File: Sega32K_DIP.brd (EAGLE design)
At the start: 65.7 x 37.9 mm, 4 parts

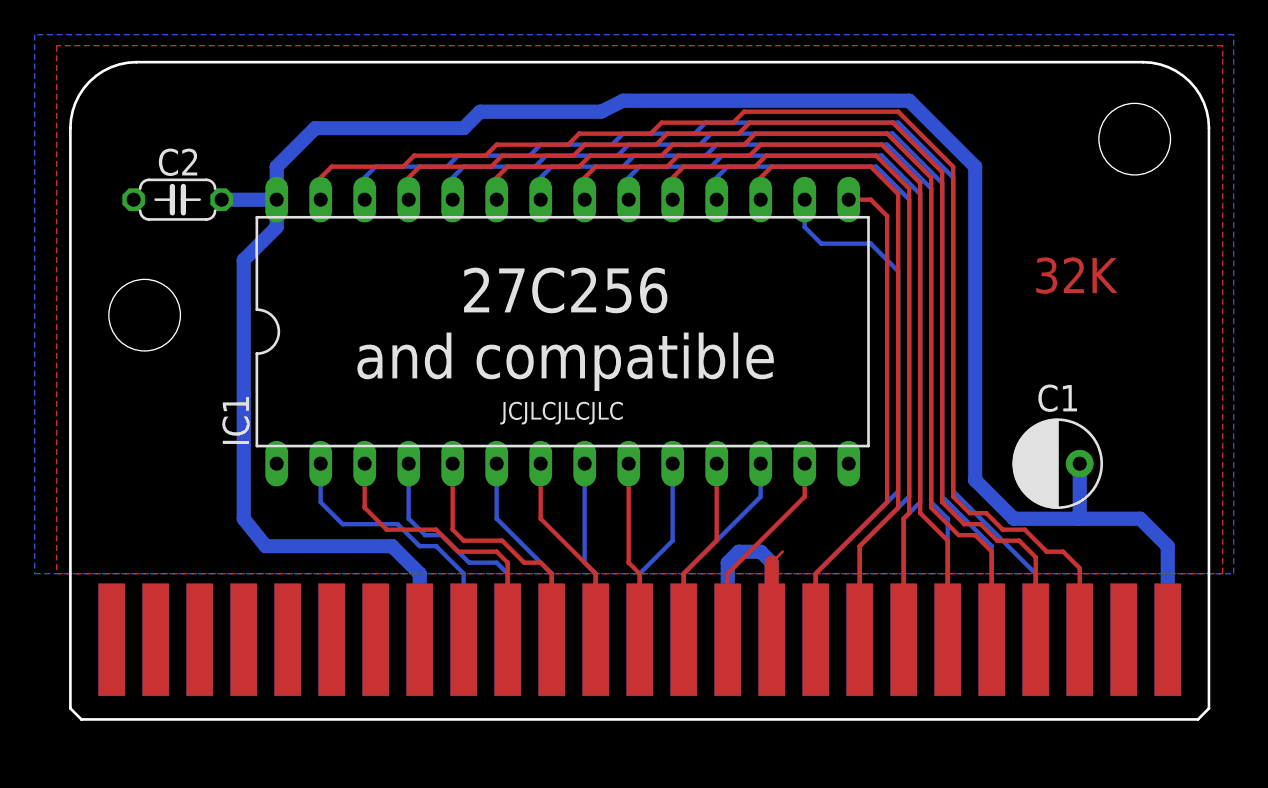
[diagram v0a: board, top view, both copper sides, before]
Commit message: Add files via upload
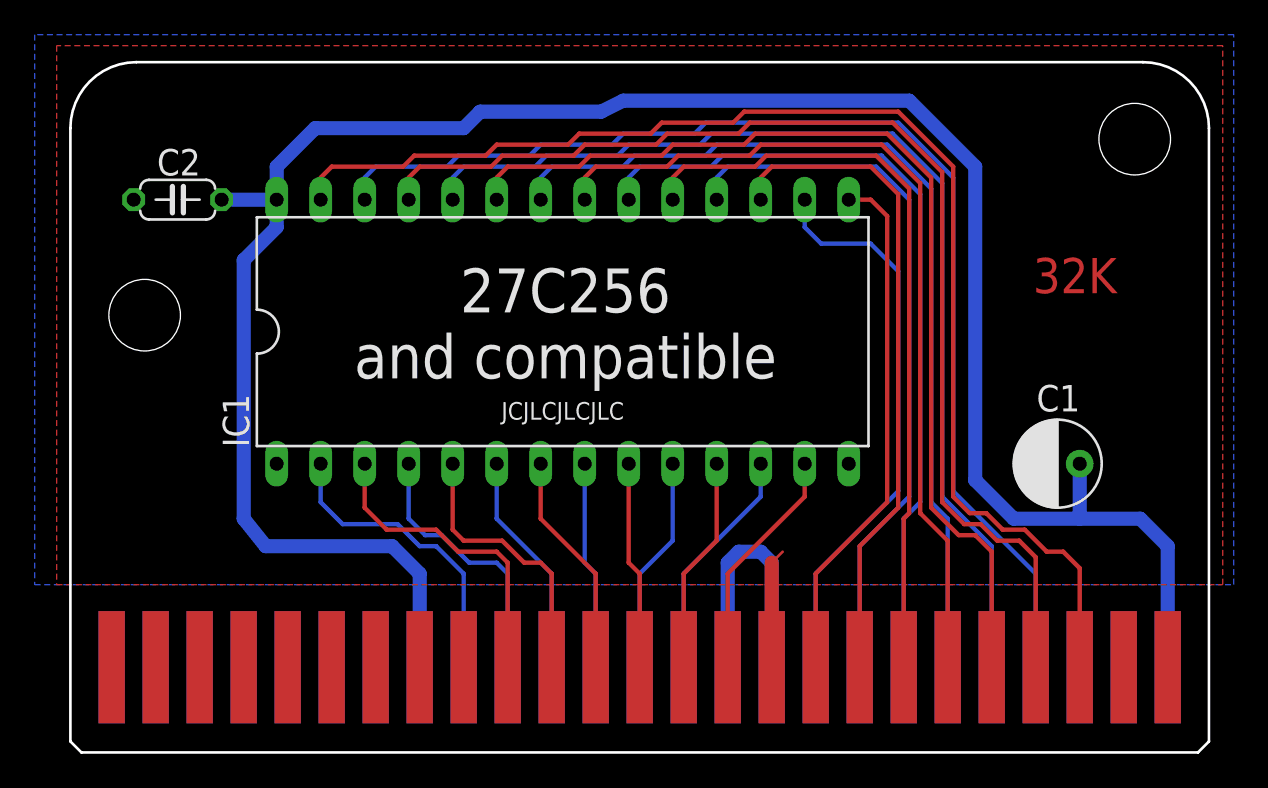
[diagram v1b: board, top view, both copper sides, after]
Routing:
- net GND: track 17.3 -> 22.1 mm
- net +5V: track 122.4 -> 125.6 mm
- net D5: track 36.8 -> 38.4 mm
- net A9: track 59.3 -> 60.9 mm
- net A14: track 72.9 -> 74.5 mm
- net A13: track 66.5 -> 68.1 mm
- net A11: track 57.1 -> 58.7 mm
- net D2: track 12.0 -> 13.6 mm
- net D1: track 12.0 -> 13.6 mm
- net D0: track 10.9 -> 12.5 mm
- net A6: track 14.0 -> 15.6 mm
- net A5: track 14.4 -> 16.0 mm
- net A4: track 11.5 -> 13.1 mm
- net A3: track 11.5 -> 13.1 mm
- net A2: track 10.4 -> 12.0 mm
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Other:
- board size 65.7 x 37.9 mm -> 65.7 x 39.8 mm
